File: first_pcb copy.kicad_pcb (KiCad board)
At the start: 2 copper layers, 260.6 x 176.8 mm, 20 parts, among them U1 NE555P, U2 4017

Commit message: updated files
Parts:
- moved D10 187.1 mm to (239.3, 126.2)
- moved D6 146.7 mm to (104.6, 177.5)
- moved D7 113.8 mm to (83.6, 160.0)
- moved D5 105.7 mm to (126.5, 188.0)
- moved D4 97.7 mm to (159.3, 193.8), turned to 180 degrees
- moved D8 82.2 mm to (66.3, 137.4)
- moved D3 78.7 mm to (191.5, 183.6), turned to 180 degrees
- moved D2 54.7 mm to (213.1, 168.7), turned to 180 degrees
- moved D9 51.1 mm to (59.9, 115.3)
- moved C4 42.4 mm to (165.9, 25.9)
- moved RV1 42.4 mm to (140.5, 31.0)
- moved U1 42.4 mm to (176.0, 51.3)
- moved C3 42.4 mm to (148.6, 25.9)
- moved R1 42.4 mm to (143.0, 41.1)
- moved R4 42.4 mm to (132.8, 51.3)
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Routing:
- net Net-(D4-A): track 332.5 -> 148.0 mm
- net Net-(D10-A): track 235.1 -> 87.5 mm, vias 0 -> 1
- net Net-(D5-A): track 262.4 -> 159.2 mm, vias 2 -> 1
- net Net-(D1-K): track 526.8 -> 443.5 mm, vias 2 -> 0
- net Net-(D8-A): track 238.5 -> 172.2 mm, vias 0 -> 3
- net OUT: track 198.4 -> 132.2 mm
- net Net-(D6-A): track 85.9 -> 146.0 mm
- net +5V: track 168.4 -> 119.9 mm
- net Net-(D1-A): track 46.8 -> 86.3 mm
- net GND: track 322.1 -> 284.2 mm
- net Net-(D2-A): track 72.7 -> 100.8 mm
- net Net-(D9-A): track 196.9 -> 177.5 mm, vias 0 -> 2
- net Net-(D7-A): track 177.7 -> 187.4 mm, vias 0 -> 2
- net Net-(D3-A): track 117.9 -> 119.3 mm, vias 0 -> 1
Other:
- board size 260.6 x 176.8 mm -> 197.8 x 197.8 mm
- board text added: "Jake Hopkins 1-10-25"

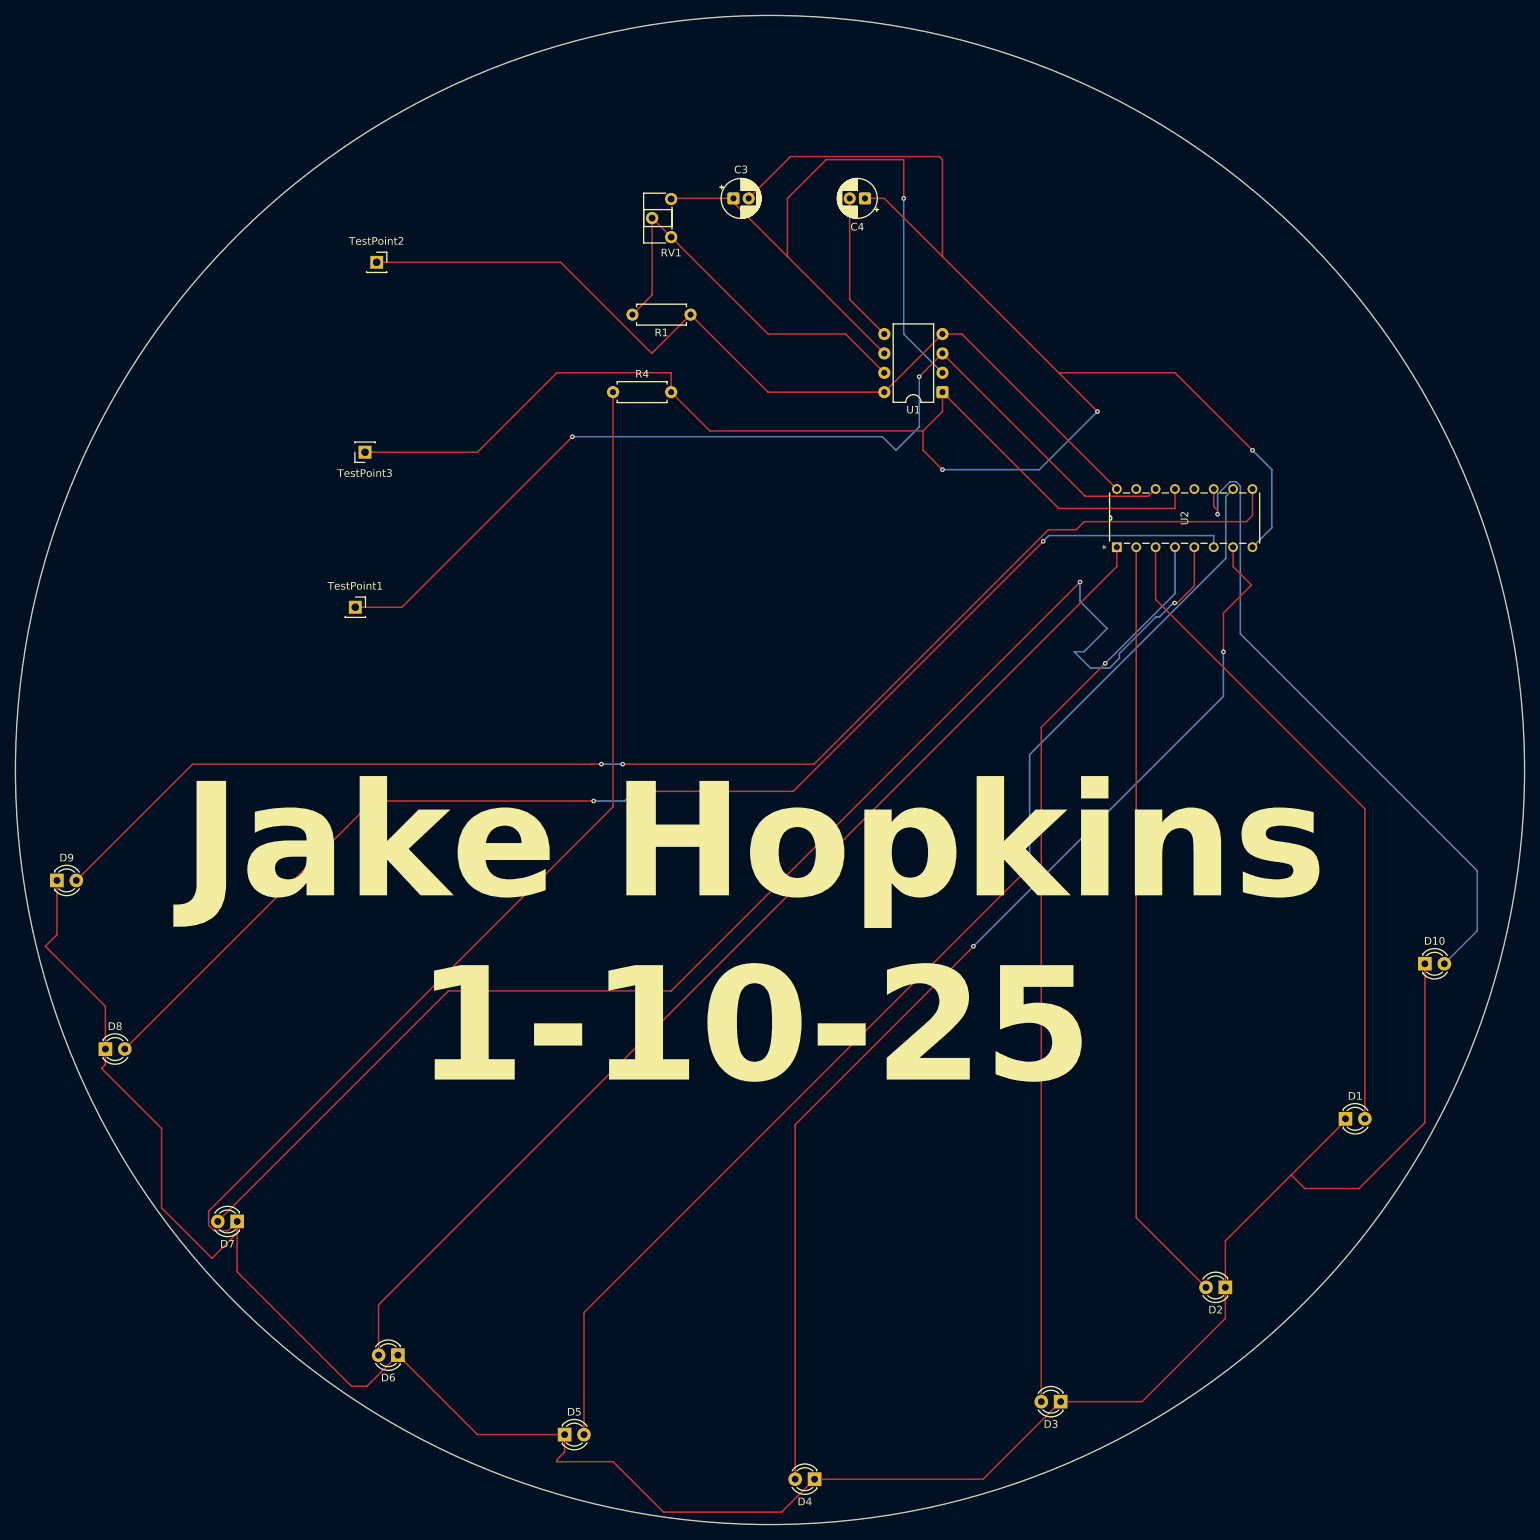
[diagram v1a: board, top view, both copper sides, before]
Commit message: added more files
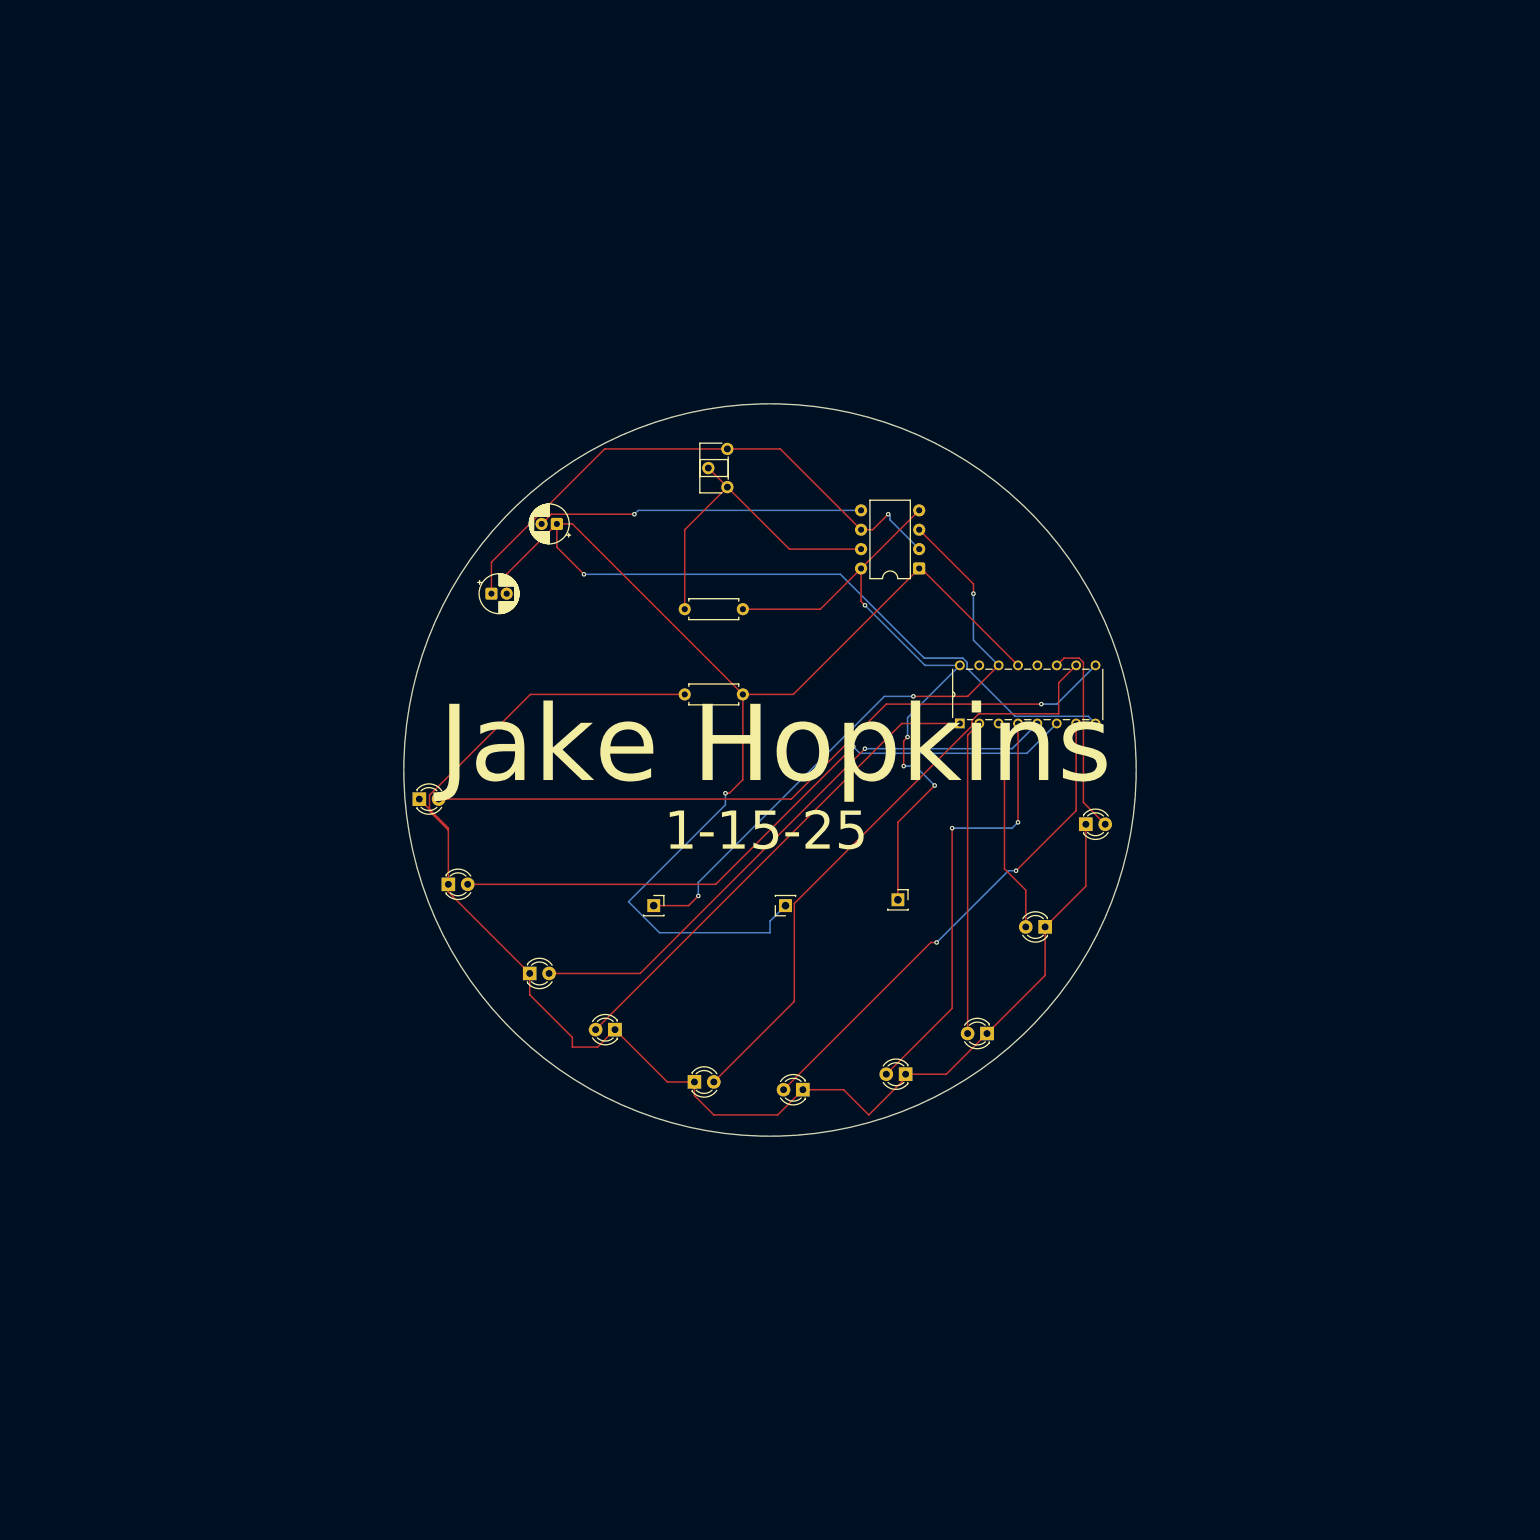
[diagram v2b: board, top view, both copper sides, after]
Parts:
- moved TestPoint2 107.9 mm to (170.2, 117.9)
- moved TestPoint3 81.1 mm to (155.4, 118.6)
- moved C3 60.8 mm to (116.9, 77.7)
- moved C4 58.8 mm to (125.5, 68.6)
- moved TestPoint1 55.3 mm to (138.2, 118.6)
- moved D6 51.3 mm to (133.1, 134.9)
- moved D4 51.1 mm to (157.7, 142.7)
- moved D7 50.3 mm to (121.9, 127.5), turned to 0 degrees
- moved D8 49.9 mm to (111.3, 115.8)
- moved D5 49.3 mm to (143.5, 141.7)
- moved D9 48.7 mm to (107.4, 104.6)
- moved D10 48.1 mm to (194.8, 108.0)
- moved D3 47.5 mm to (171.2, 140.7)
- moved D1 46.7 mm to (189.5, 121.4), turned to 180 degrees
- moved D2 45.6 mm to (181.9, 135.4)
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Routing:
- net Net-(D1-K): track 443.5 -> 186.6 mm
- net Net-(D7-A): track 187.4 -> 77.6 mm, vias 2 -> 1
- net Net-(D8-A): track 172.2 -> 86.7 mm, vias 3 -> 1
- net Net-(D9-A): track 177.5 -> 93.4 mm, vias 2 -> 1
- net Net-(D4-A): track 148.0 -> 64.9 mm
- net Net-(D6-A): track 146.0 -> 64.4 mm
- net Net-(D5-A): track 159.2 -> 80.4 mm, vias 1 -> 0
- net Net-(D3-A): track 119.3 -> 57.7 mm, vias 1 -> 2
- net Net-(D10-A): track 87.5 -> 26.5 mm, vias 1 -> 0
- net Net-(D2-A): track 100.8 -> 41.3 mm
- net Net-(D1-A): track 86.3 -> 28.1 mm
- net OUT: track 132.2 -> 81.4 mm, vias 2 -> 3
- net GND: track 284.2 -> 235.7 mm, vias 3 -> 2
- net +5V: track 119.9 -> 87.6 mm, vias 0 -> 4
- net Net-(U1-CV): track 19.7 -> 42.6 mm, vias 0 -> 1
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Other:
- board size 197.8 x 197.8 mm -> 96 x 96 mm
- board text added: "1-15-25"
- board text added: "First PCB"
- board text added: "Jake Hopkins"
- board text removed: "Jake Hopkins 1-10-25"
